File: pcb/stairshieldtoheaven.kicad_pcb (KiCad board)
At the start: 2 copper layers, 105.4 x 97.8 mm, 30 parts, among them P1 CONN_10X2, P10 5, P11 6, P12 7, P13 8, P14 9, P15 10, P16 11, P17 12, P18 13, P19 14, P2 LED1, P20 15, P21 16, P22 17, P23 18, P24 19, P25 20, P4 5V, P5 1, P6 2, P7 3, P8 4, P9 12V

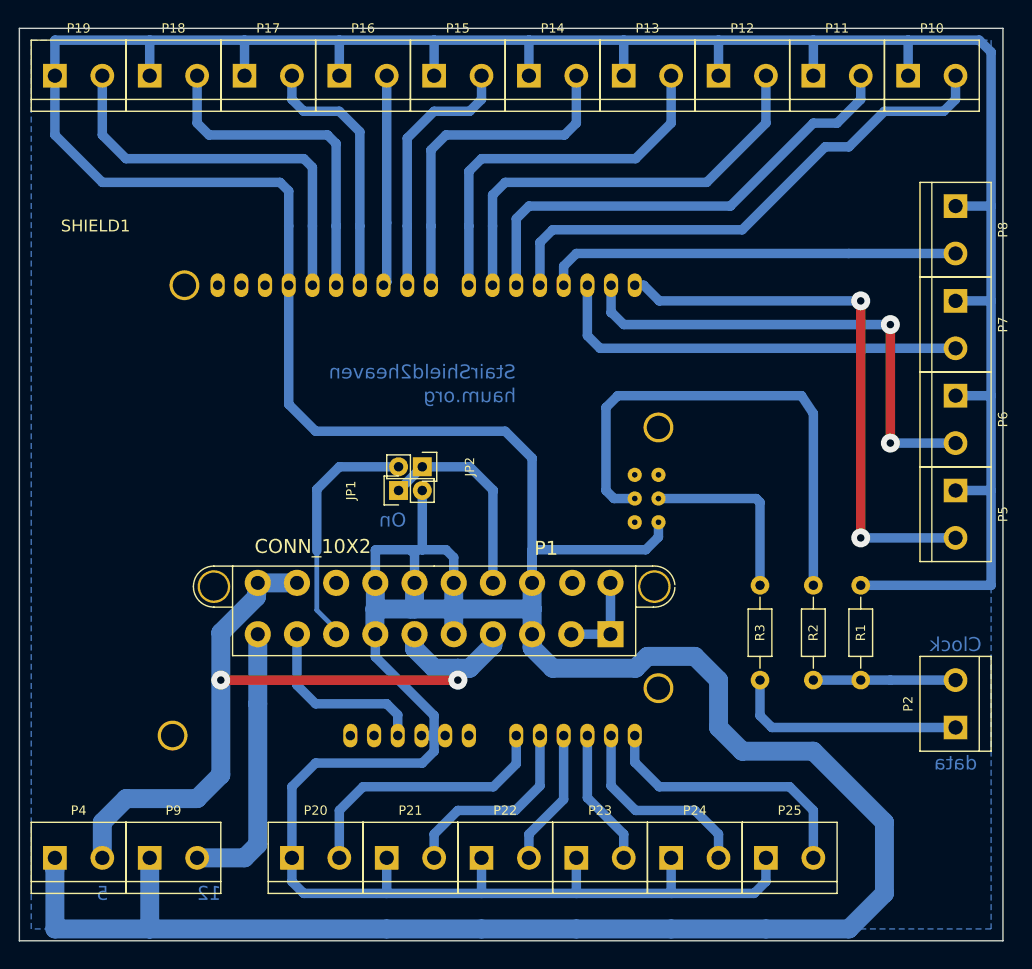
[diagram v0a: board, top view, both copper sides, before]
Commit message: Add missing PCB update
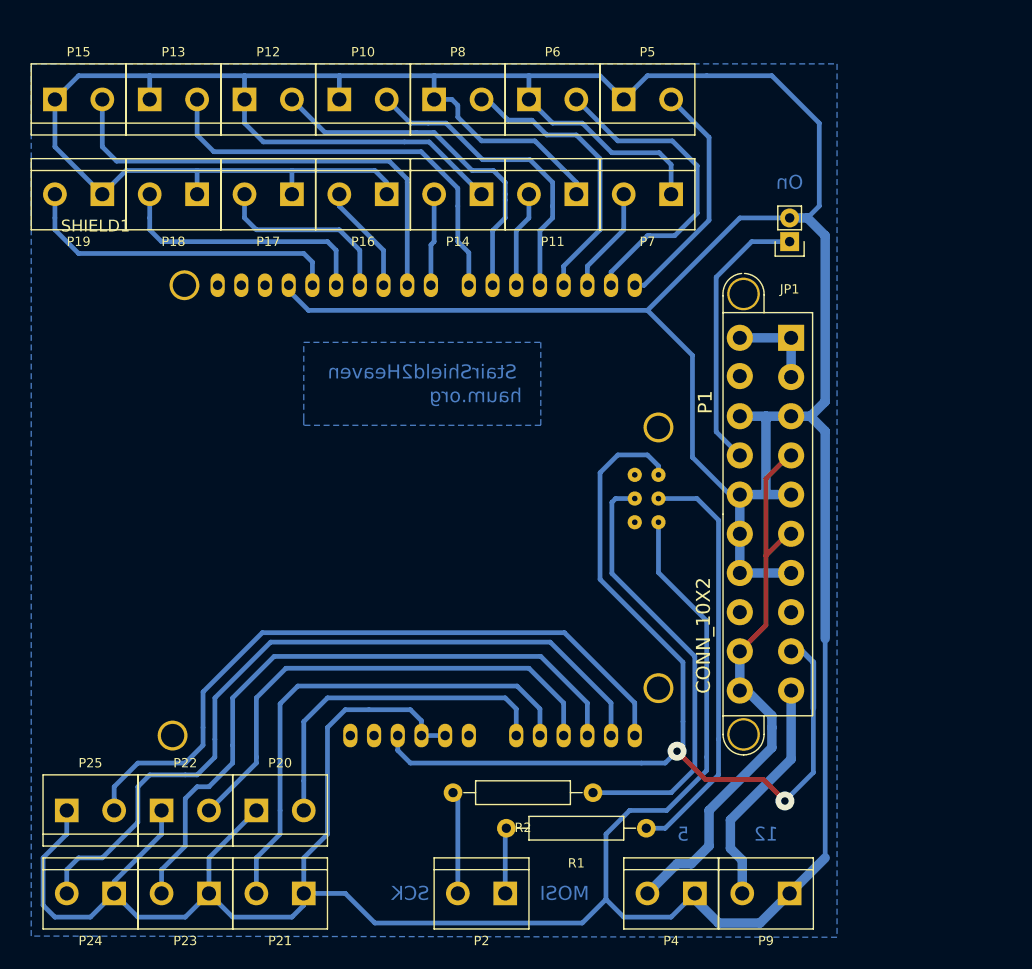
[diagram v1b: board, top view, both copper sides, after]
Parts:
- removed JP2: JUMPER, Pin_Headers:Pin_Header_Straight_1x02
- removed R3: RL, Resistors_ThroughHole:Resistor_Horizontal_RM10mm
- R1: value RPLD -> R; footprint Resistors_ThroughHole:Resistor_Horizontal_RM10mm -> Resistors_ThroughHole:Resistor_Horizontal_RM15mm
- R2: value RL -> R; footprint Resistors_ThroughHole:Resistor_Horizontal_RM10mm -> Resistors_ThroughHole:Resistor_Horizontal_RM15mm
- moved P25 75.1 mm to (82.5, 102.9)
- moved P24 64.9 mm to (82.5, 111.8), turned to 180 degrees
- moved P4 63.6 mm to (144.8, 111.8), turned to 180 degrees
- moved P9 63.6 mm to (154.9, 111.8), turned to 180 degrees
- moved P10 61.0 mm to (111.8, 26.7)
- moved P5 55.4 mm to (142.2, 26.7), turned to 0 degrees
- moved P8 55.1 mm to (121.9, 26.7), turned to 0 degrees
- moved P6 55.1 mm to (132.1, 26.7), turned to 0 degrees
- moved P2 54.7 mm to (124.5, 111.8), turned to 180 degrees
- moved P12 50.9 mm to (101.6, 26.7)
- moved P13 50.9 mm to (91.4, 26.7)
- moved JP1 49.7 mm to (157.5, 41.9), turned to 180 degrees
- moved P23 44.6 mm to (92.7, 111.8), turned to 180 degrees
- moved P15 40.7 mm to (81.3, 26.7)
- moved R1 37.0 mm to (134.6, 104.8), turned to 180 degrees
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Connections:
- net /clock renamed /SCK
- net Net-(SHIELD1-Pad_MIS) renamed /MISO
- net Net-(SHIELD1-Pad_RST) renamed /Reset
- P1 pad 17: /5V_SB -> VCC
- R1 pad 1: Net-(P2-Pad2) -> /MOSI
- R1 pad 2: GND -> Net-(P2-Pad1)
- SHIELD1 pad 5V: /5V_SB -> VCC
- SHIELD1 pad _5V: Net-(SHIELD1-Pad_5V) -> VCC
- SHIELD1 pad _MOS: /data -> /MOSI
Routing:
- net VCC: track 0.00 -> 107.6 mm, vias 0 -> 2
- net /19: track 21.6 -> 83.1 mm
- net /18: track 14.7 -> 70.3 mm
- net /20: track 29.2 -> 76.4 mm
- net /MOSI: track 0.00 -> 44.8 mm
- net GND: track 684.4 -> 641.6 mm
- net /6: track 51.9 -> 10.3 mm
- net /17: track 14.6 -> 53.6 mm
- net /1: track 60.5 -> 25.5 mm, vias 2 -> 0
- net /3: track 45.4 -> 11.4 mm
- net /16: track 21.4 -> 53.9 mm
- net /9: track 36.3 -> 9.90 mm
- net /PG: track 26.1 -> 0.00 mm
- net /5: track 58.0 -> 33.0 mm
- net /5V: track 84.7 -> 61.6 mm, vias 2 -> 0
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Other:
- board outline removed
- net class Default: clearance 0.254 -> 0.5; trace_width 0.254 -> 0.6
- net class piste_cmd: clearance 0.254 -> 0.5
- net class piste_cmdS: clearance 0.254 -> 0.5
- net class piste_pwr: clearance 0.254 -> 0.5
- rule trace_clearance: 0.254 -> 0.5
- board text added: "MOSI"
- board text added: "SCK"
- board text added: "StairShield2Heaven"
- board text removed: "Clock"
- board text removed: "StairShield2heaven"
- board text removed: "data"
